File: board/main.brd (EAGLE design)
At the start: 40 x 30.4 mm, 13 parts, among them Q1 12MHz, U1 ATMEGA328P_TQFP

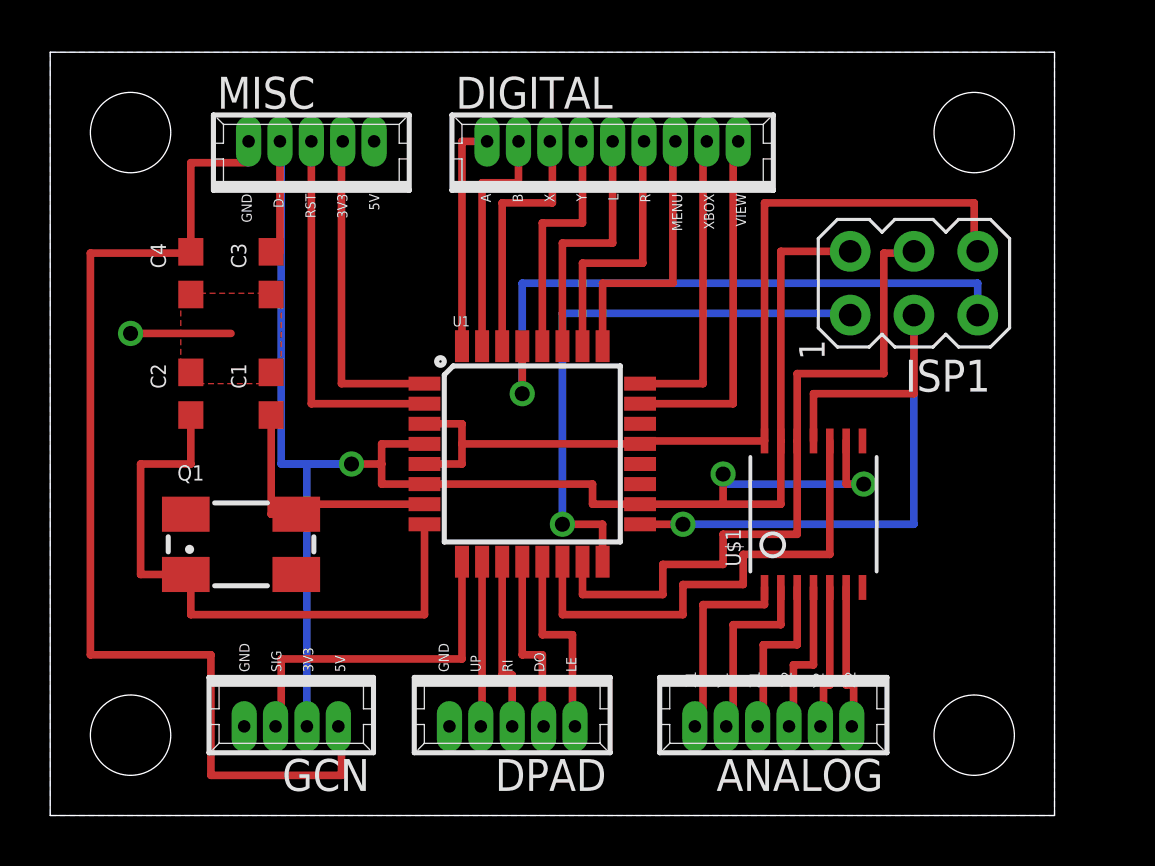
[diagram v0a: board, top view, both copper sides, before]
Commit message: Ready to order v0.2 boards
Signed-off-by: Garrett Greenwood <garrettagreenwood@gmail.com>
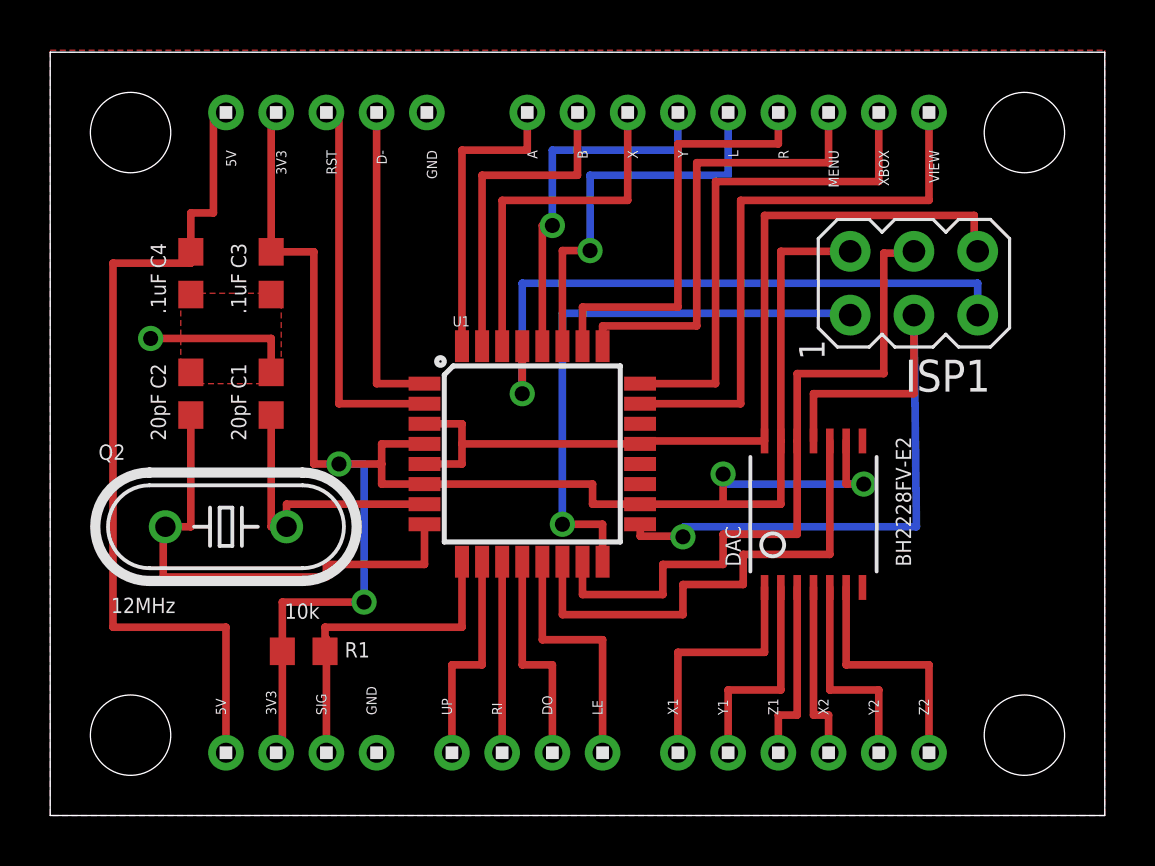
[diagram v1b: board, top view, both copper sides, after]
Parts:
- removed DIGITAL: 53047-09, con-molex:53047-09
- removed Q1: 12MHz, crystal:CTS406
- added Q2: 12MHz, crystal:HC49/S
- added R1: 10k, resistor:R0603
- added U$6: 1X9, headers(2mm):1X9
- ANALOG: value 53047-06 -> 1X6; device con-molex:53047-06 -> headers(2mm):1X6
- DPAD: value 53047-05 -> 1X4; device con-molex:53047-05 -> headers(2mm):1X4
- GCN: value 53047-04 -> 1X4; device con-molex:53047-04 -> headers(2mm):1X4
- MISC: value 53047-05 -> 1X5; device con-molex:53047-05 -> headers(2mm):1X5
- moved ANALOG 1.92 mm to (30.0, 2.50), turned to 0 degrees
- moved MISC 1.71 mm to (11.0, 28.0)
- moved DPAD 1.62 mm to (19.0, 2.50), turned to 0 degrees
- moved GCN 1.55 mm to (10.0, 2.50)
- renumbered U$1 to DAC
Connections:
- net XBOX_RESET renamed MISC-RST
- removed net D_DOWN: DPAD.4, U1.12
- removed net D_LEFT: DPAD.5, U1.13
- removed net D_RIGHT: DPAD.3, U1.11
- removed net D_UP: DPAD.2, U1.10
- removed net USB_D-: MISC.2, U1.1
- new net DPAD-D: DPAD.3, U1.12
- new net DPAD-L: DPAD.4, U1.13
- new net DPAD-R: DPAD.2, U1.11
- new net DPAD-U: DPAD.1, U1.10
- new net MISC-D-: MISC.4, U1.1
- net 3V3: now also MISC.2, R1.2; no longer MISC.4
- net 5V: now also MISC.1; no longer MISC.5
- net A: now also U$6.9; no longer DIGITAL.1
- net B: now also U$6.8; no longer DIGITAL.2
- net GCN_SIG: now also R1.1
- net GND: now also MISC.5; no longer DPAD.1, MISC.1
- net L: now also U$6.5; no longer DIGITAL.5
- net MENU: now also U$6.3; no longer DIGITAL.7
- net N$1: now also Q2.2; no longer Q1.3
- net N$2: now also Q2.1; no longer Q1.1
- net R: now also U$6.4; no longer DIGITAL.6
- net VIEW: now also U$6.1; no longer DIGITAL.9
- net X: now also U$6.7; no longer DIGITAL.3
- net XBOX: now also U$6.2; no longer DIGITAL.8
- net Y: now also U$6.6; no longer DIGITAL.4
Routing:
- net USB_D-: track 13.0 -> 0.00 mm
- net MISC-D-: track 0.00 -> 12.7 mm
- net DPAD-L: track 0.00 -> 10.0 mm
- net 5V: track 43.6 -> 34.5 mm
- net DPAD-U: track 0.00 -> 8.81 mm
- net DPAD-D: track 0.00 -> 8.81 mm
- net A: track 14.4 -> 23.1 mm
- net B: track 12.3 -> 20.3 mm
- net D_LEFT: track 7.86 -> 0.00 mm
- net DPAD-R: track 0.00 -> 7.61 mm
- net D_DOWN: track 7.41 -> 0.00 mm
- net X: track 11.1 -> 18.3 mm
- net D_RIGHT: track 6.96 -> 0.00 mm
- net D_UP: track 6.61 -> 0.00 mm
- net Y: track 10.6 -> 17.1 mm
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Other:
- board size 40 x 30.4 mm -> 42 x 30.4 mm
- board text added: "GARRETT GREENWOOD GAMECUBE->XBOX ONE ADAPTER V0.2"
- board text removed: "GARRETT GREENWOOD GAMECUBE->XBOX ONE ADAPTER V0.1"
